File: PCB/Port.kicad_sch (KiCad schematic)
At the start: 1 part, among them J13 SBH11-PBPC-D10-RA-BK

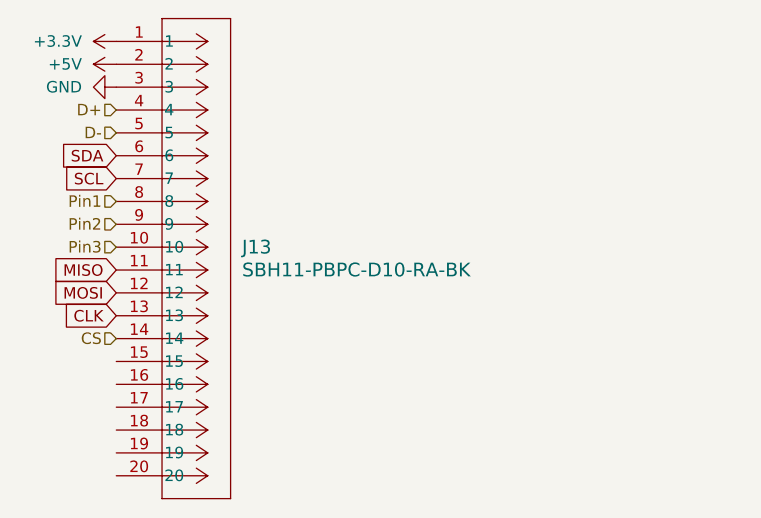
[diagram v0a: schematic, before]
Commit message: Updated PCB
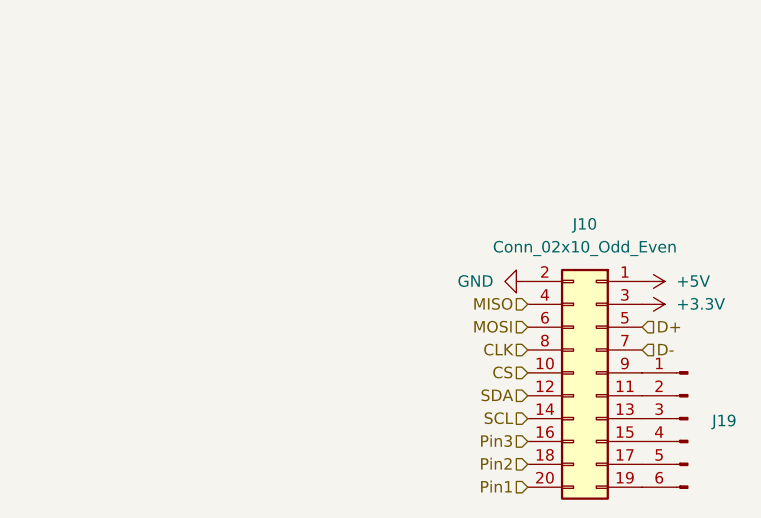
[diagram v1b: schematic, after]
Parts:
- removed J13: SBH11-PBPC-D10-RA-BK, Library:CONN20_D10-RA-BK_SUL, symbol ConnPins:SBH11-PBPC-D10-RA-BK
- added J10: Conn_02x10_Odd_Even, Connector_PinSocket_2.00mm:PinSocket_2x10_P2.00mm_Horizontal, symbol Connector_Generic:Conn_02x10_Odd_Even
- added J19: Conn_01x06_Pin, Connector_PinHeader_1.27mm:PinHeader_1x06_P1.27mm_Vertical, symbol Connector:Conn_01x06_Pin
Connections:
- net +3.3V: now also J10.3 (Pin_3)
- net +5V: now also J10.1 (Pin_1)
- net CLK: now also J10.8 (Pin_8)
- net CS: now also J10.10 (Pin_10)
- net D+: now also J10.5 (Pin_5)
- net D-: now also J10.7 (Pin_7)
- net GND: now also J10.2 (Pin_2)
- net MISO: now also J10.4 (Pin_4)
- net MOSI: now also J10.6 (Pin_6)
- net Pin1: now also J10.20 (Pin_20)
- net Pin2: now also J10.18 (Pin_18)
- net Pin3: now also J10.16 (Pin_16)
- net SCL: now also J10.14 (Pin_14)
- net SDA: now also J10.12 (Pin_12)
- new net: J10.11 (Pin_11), J19.2 (Pin_2)
- new net: J10.13 (Pin_13), J19.3 (Pin_3)
- new net: J10.15 (Pin_15), J19.4 (Pin_4)
- new net: J10.17 (Pin_17), J19.5 (Pin_5)
- new net: J10.19 (Pin_19), J19.6 (Pin_6)
- new net: J10.9 (Pin_9), J19.1 (Pin_1)
